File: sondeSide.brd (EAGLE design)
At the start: 105.2 x 31.8 mm, 41 parts

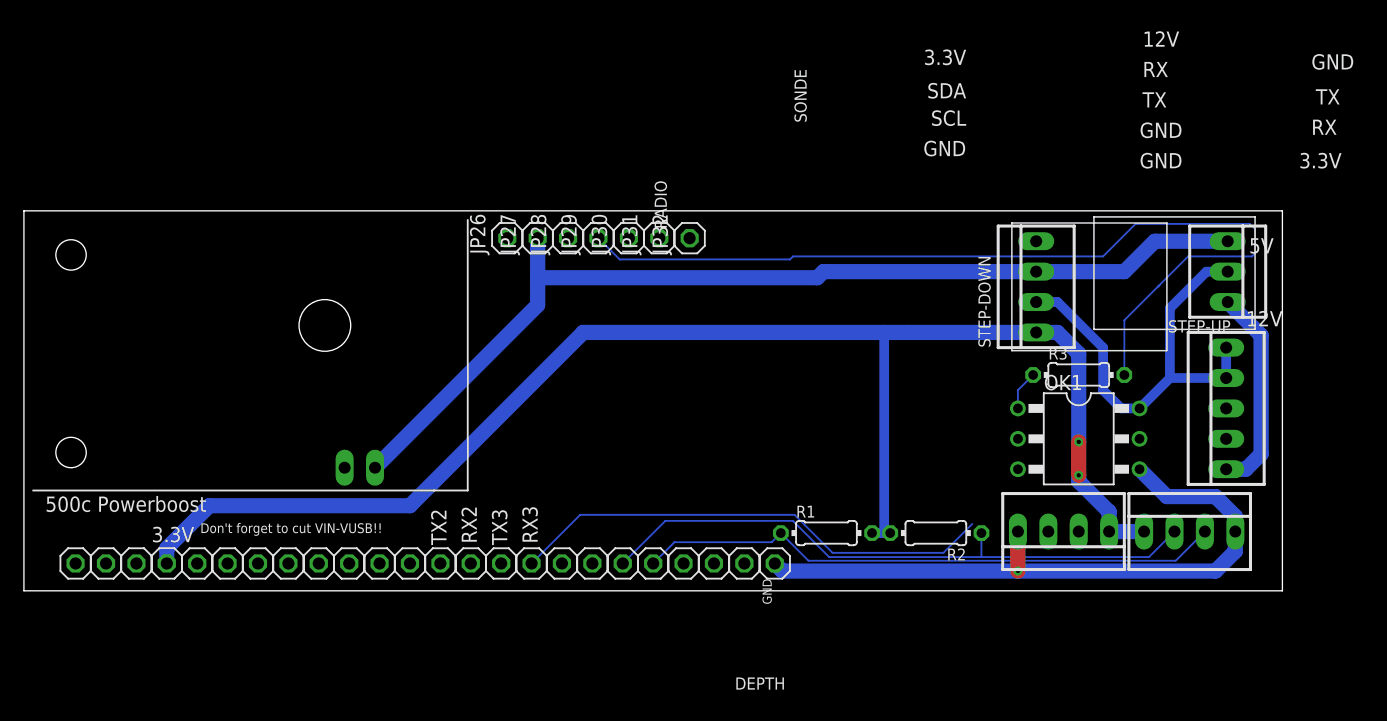
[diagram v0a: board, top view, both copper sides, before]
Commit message: Good to go! Just place labels
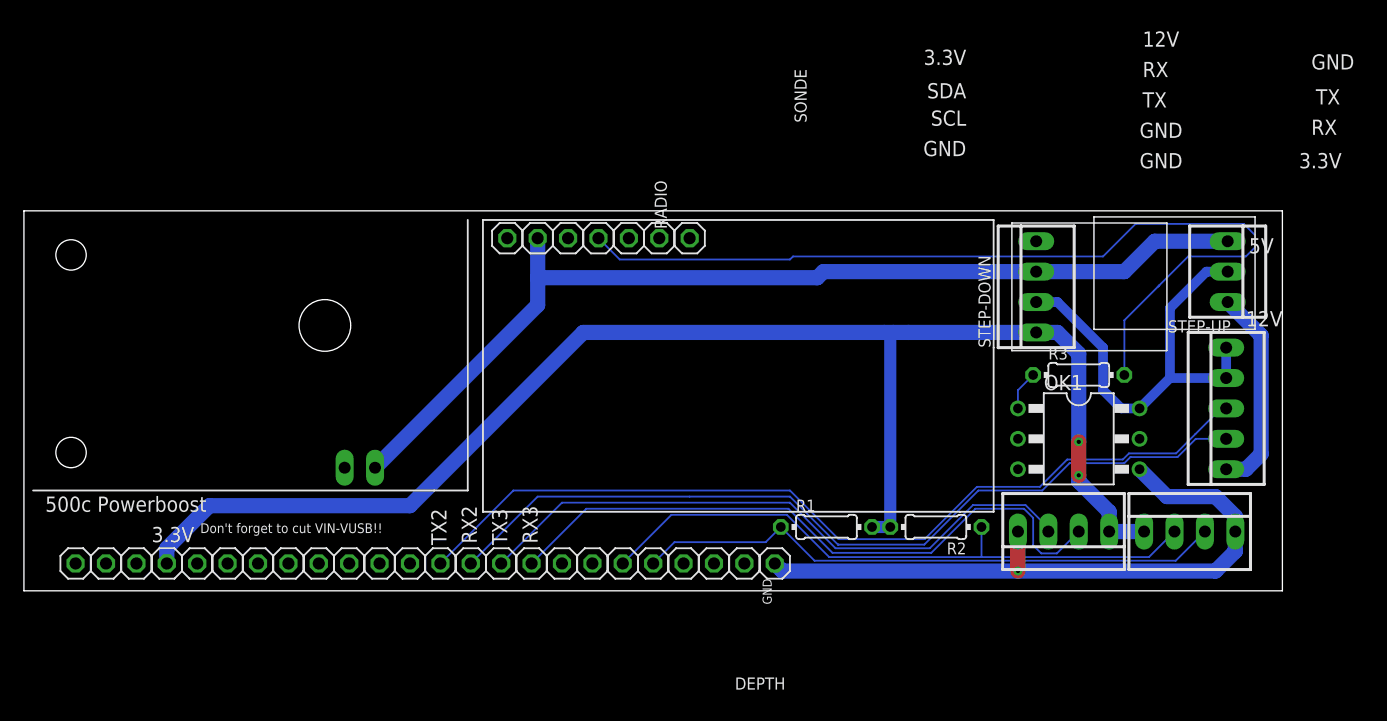
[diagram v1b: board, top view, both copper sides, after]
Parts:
- moved R1 0.51 mm to (67.1, 5.33)
- moved R2 0.51 mm to (76.2, 5.33)
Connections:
- net RX2: now also SONDE.2; no longer RADIO.2
- net RX3: now also RADIO.2; no longer SONDE.2
- net TX2: now also SONDE.3; no longer RADIO.3
- net TX3: now also RADIO.3; no longer SONDE.3
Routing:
- net TX2: track 0.00 -> 74.4 mm
- net RX2: track 0.00 -> 70.8 mm
- net TX3: track 0.00 -> 52.0 mm
- net RX3: track 40.8 -> 54.3 mm
- net SDA: track 51.7 -> 52.6 mm
- net 3.3V: track 126.7 -> 125.9 mm
- net D1: track 77.0 -> 76.4 mm
